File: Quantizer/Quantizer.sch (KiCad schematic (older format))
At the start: 43 parts, among them J1 EuroPower, J2 CV, J3 Gate, J4 IN1, SW1 Reset, U1 L7805, U2 TL082

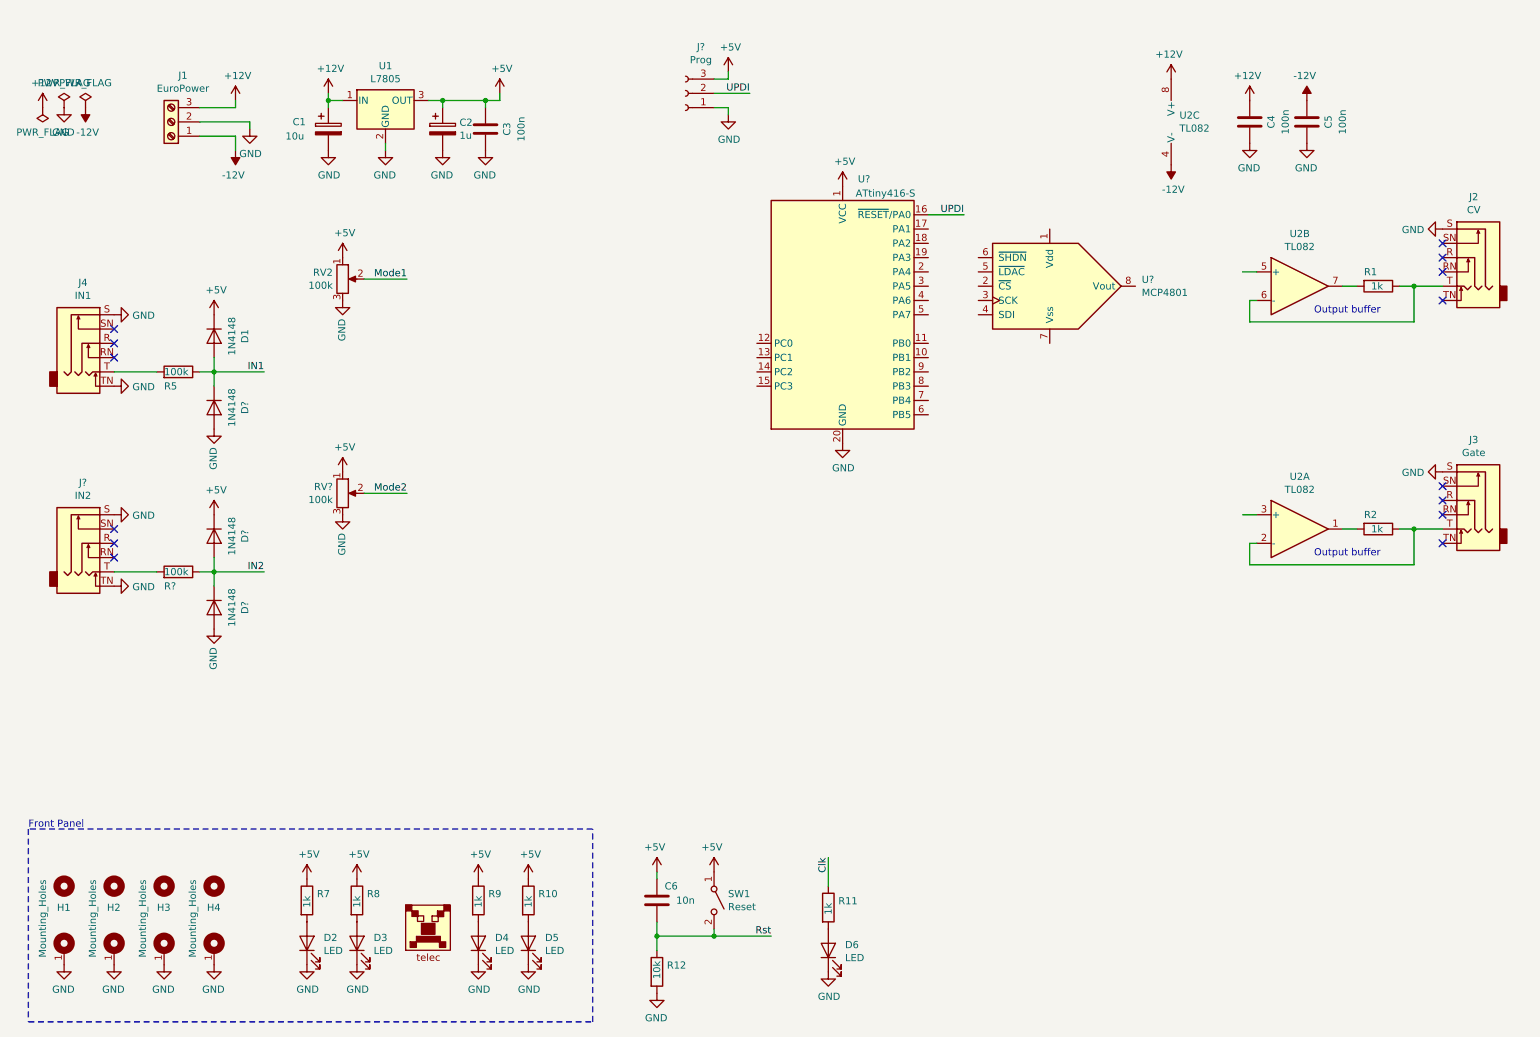
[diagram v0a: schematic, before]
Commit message: Quantizer layout done!
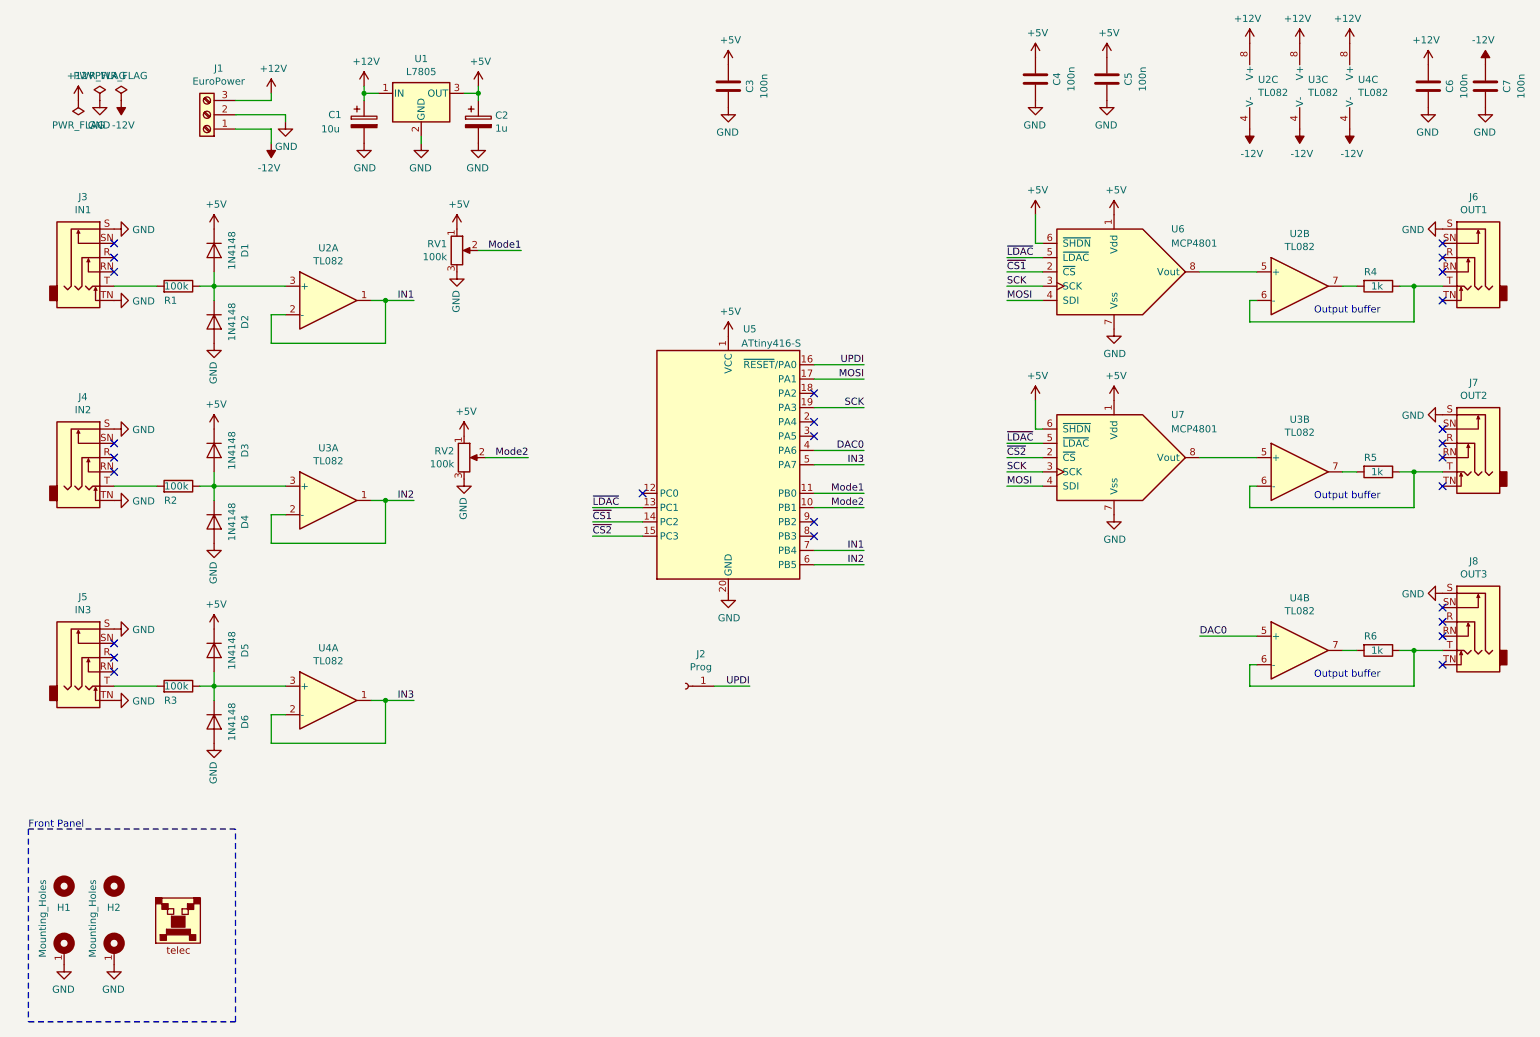
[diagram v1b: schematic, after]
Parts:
- removed C6: 10n, Capacitor_THT:C_Disc_D7.0mm_W2.5mm_P5.00mm, symbol Device:C
- removed D2, D3, D4, D5: LED, LED_SMD:LED_1206_3216Metric_Castellated, symbol Device:LED
- removed D6: LED, LED_SMD:LED_1206_3216Metric_ReverseMount_Hole1.8x2.4mm, symbol Device:LED
- removed H3, H4: Mounting_Holes, Kosmo_panel:Kosmo_Panel_Dual_Mounting_Holes, symbol Kosmo:Mounting_Holes
- removed J?: Prog, symbol Connector:Conn_01x03_Female
- removed R10, R11, R7, R8, R9: 1k, Resistor_SMD:R_1206_3216Metric_Pad1.42x1.75mm_HandSolder, symbol Device:R
- removed R12: 10k, Resistor_THT:R_Axial_DIN0204_L3.6mm_D1.6mm_P7.62mm_Horizontal, symbol Device:R
- removed SW1: Reset, Button_Switch_THT:SW_PUSH_6mm, symbol Switch:SW_SPST
- added C4, C5: 100n, Capacitor_SMD:C_1206_3216Metric_Pad1.42x1.75mm_HandSolder, symbol Device:C
- added D5, D6: 1N4148, Diode_SMD:D_1206_3216Metric_Pad1.42x1.75mm_HandSolder, symbol Diode:1N4148
- added J2: Prog, TestPoint:TestPoint_Pad_D2.5mm, symbol Connector:Conn_01x01_Female
- added J5: IN3, telec:JackHole, symbol Connector:AudioJack3_Switch
- added J8: OUT3, telec:JackHole, symbol Connector:AudioJack3_Switch
- added R3: 100k, Resistor_SMD:R_1206_3216Metric_Pad1.42x1.75mm_HandSolder, symbol Device:R
- added R6: 1k, Resistor_SMD:R_1206_3216Metric_Pad1.42x1.75mm_HandSolder, symbol Device:R
- added unit 1 of U2
- added unit 3 of U2
- added unit 1 of U3
- added unit 3 of U3
- added unit 2 of U4
- added unit 1 of U4
- added U7: MCP4801, Package_DIP:DIP-8_W7.62mm, symbol Analog_DAC:MCP4801
- C1, C2: footprint Capacitor_THT:CP_Radial_D8.0mm_P3.80mm -> Capacitor_THT:CP_Radial_D4.0mm_P1.50mm
- C3: footprint Capacitor_THT:C_Disc_D7.0mm_W2.5mm_P5.00mm -> Capacitor_SMD:C_1206_3216Metric_Pad1.42x1.75mm_HandSolder
- C6: renamed from C4; footprint Capacitor_THT:C_Disc_D7.0mm_W2.5mm_P5.00mm -> Capacitor_SMD:C_1206_3216Metric_Pad1.42x1.75mm_HandSolder
- C7: renamed from C5; footprint Capacitor_THT:C_Disc_D7.0mm_W2.5mm_P5.00mm -> Capacitor_SMD:C_1206_3216Metric_Pad1.42x1.75mm_HandSolder
- D1: footprint Diode_THT:D_DO-35_SOD27_P7.62mm_Horizontal -> Diode_SMD:D_1206_3216Metric_Pad1.42x1.75mm_HandSolder
- D2, D3, D4: renamed from D?; footprint Diode_THT:D_DO-35_SOD27_P7.62mm_Horizontal -> Diode_SMD:D_1206_3216Metric_Pad1.42x1.75mm_HandSolder
- J6: renamed from J2; value CV -> OUT1
- J7: renamed from J3; value Gate -> OUT2
- LOGO1: footprint logo:telec-32 -> logo:telec-8
- R1: renamed from R5; footprint Resistor_THT:R_Axial_DIN0204_L3.6mm_D1.6mm_P7.62mm_Horizontal -> Resistor_SMD:R_1206_3216Metric_Pad1.42x1.75mm_HandSolder
- R2: renamed from R?; footprint Resistor_THT:R_Axial_DIN0204_L3.6mm_D1.6mm_P7.62mm_Horizontal -> Resistor_SMD:R_1206_3216Metric_Pad1.42x1.75mm_HandSolder
- R4: renamed from R1; footprint Resistor_THT:R_Axial_DIN0204_L3.6mm_D1.6mm_P7.62mm_Horizontal -> Resistor_SMD:R_1206_3216Metric_Pad1.42x1.75mm_HandSolder
- R5: renamed from R2; footprint Resistor_THT:R_Axial_DIN0204_L3.6mm_D1.6mm_P7.62mm_Horizontal -> Resistor_SMD:R_1206_3216Metric_Pad1.42x1.75mm_HandSolder
- RV1: renamed from RV2; footprint Potentiometer_THT:Potentiometer_Piher_T-16L_Single_Vertical_Hole -> Potentiometer_THT:Potentiometer_Alps_RK09K_Single_Vertical
- RV2: renamed from RV?; footprint Potentiometer_THT:Potentiometer_Piher_T-16L_Single_Vertical_Hole -> Potentiometer_THT:Potentiometer_Alps_RK09K_Single_Vertical
- U1: footprint Package_TO_SOT_THT:TO-220-3_Horizontal_TabDown -> Package_TO_SOT_THT:TO-220-3_Vertical
- U2: footprint Package_DIP:DIP-8_W7.62mm_LongPads -> Package_SO:SOIC-8_3.9x4.9mm_P1.27mm
- U3, U4: renamed from U2; footprint Package_DIP:DIP-8_W7.62mm_LongPads -> Package_SO:SOIC-8_3.9x4.9mm_P1.27mm
- U6: renamed from U?; footprint (none) -> Package_DIP:DIP-8_W7.62mm
- gave numbers to parts that had none: 2
- renumbered J4 to J3
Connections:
- net labels added: DAC0, IN3, MOSI, SCK, ~CS1, ~CS2, ~LDAC
- net labels removed: Clk, Rst
- wire segments 57 -> 97
- no-connect marks 14 -> 27
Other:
- moved on the sheet: C1, C2, C6, C7, D1, D2, D3, D4, J1, J3, J4, J7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
